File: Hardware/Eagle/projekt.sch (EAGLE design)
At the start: 141 parts, among them IC1 MEGA16-P, IC2 7805T, IC3 74LS157N, Q1 BC807-40SMD, Q10 2N2222, Q11 2N2222, Q12 2N2222, Q13 BC807-40SMD, Q14 BC807-40SMD, Q15 BC807-40SMD, Q16 BC807-40SMD, Q17 BC807-40SMD, Q18 BC807-40SMD, Q19 BC807-40SMD, Q2 BC807-40SMD, Q20 2N2222, Q22 2N2222, Q24 2N2222, Q26 2N2222, Q27 2N2222, Q29 2N2222, Q3 BC807-40SMD, Q30 2N2222, Q4 BC807-40SMD, Q5 BC807-40SMD, Q6 2N2222, Q7 2N2222, Q8 2N2222, Q9 2N2222

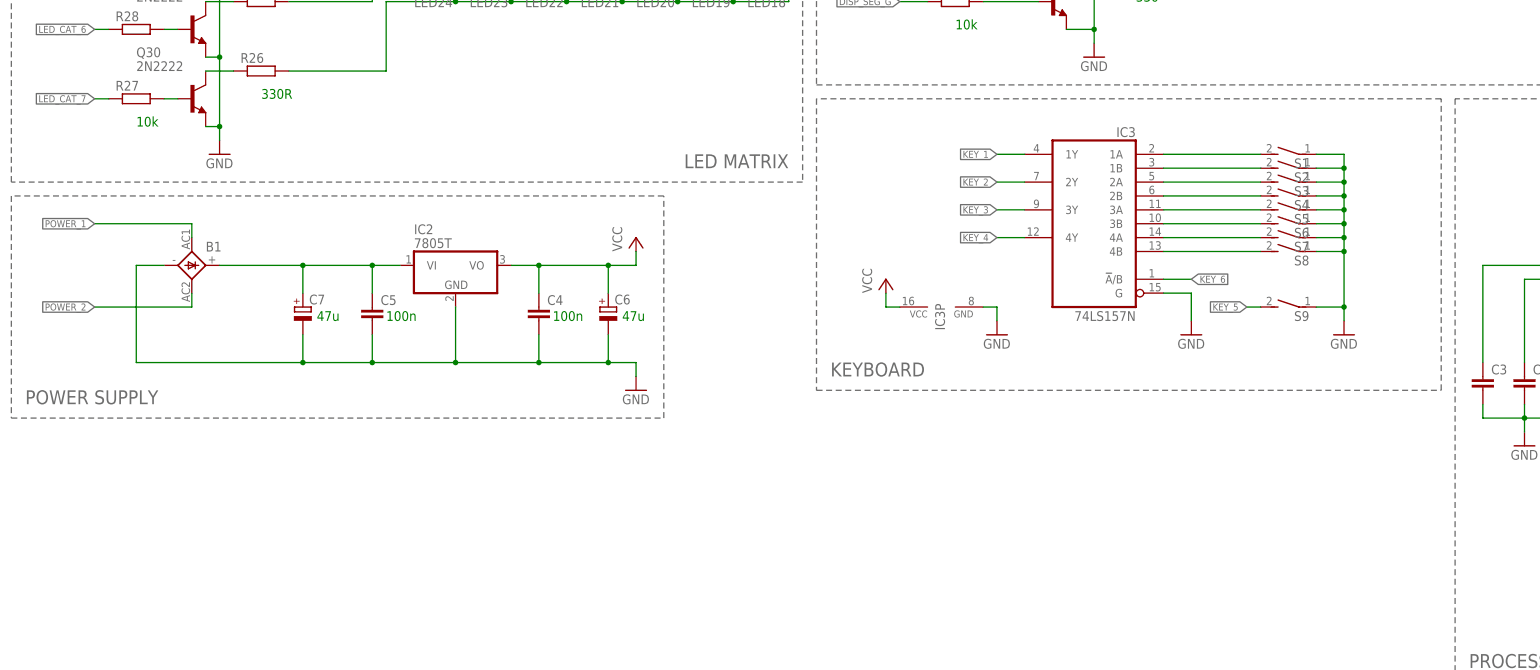
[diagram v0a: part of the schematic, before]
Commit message: przerwania, multiplekser
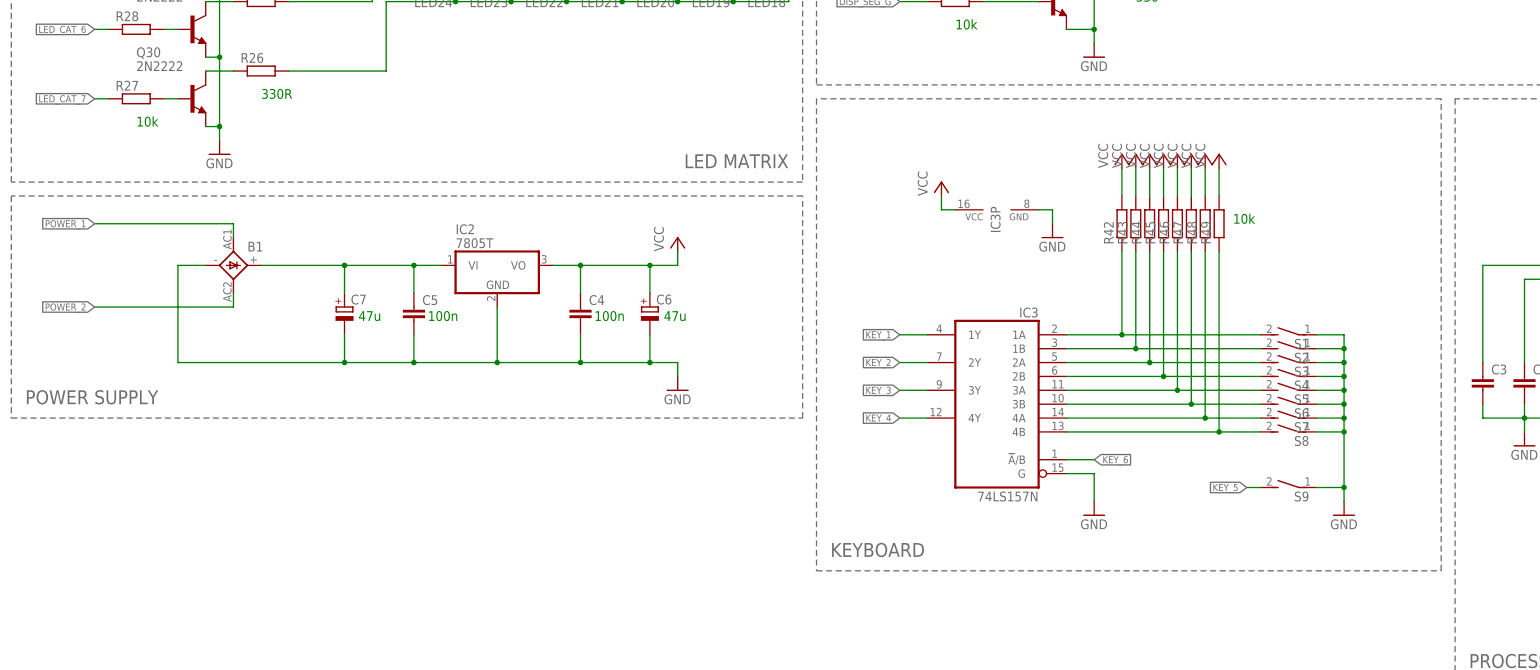
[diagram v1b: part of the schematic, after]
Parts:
- added R42, R43, R44, R45, R46, R47, R48, R49: (no value), resistor:R-EU_R0805
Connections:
- net N$27: now also R43.1
- net N$28: now also R44.1
- net N$29: now also R45.1
- net N$30: now also R46.1
- net N$31: now also R47.1
- net N$32: now also R48.1
- net N$33: now also R49.1
- net N$7: now also R42.1
- net VCC: now also R42.2, R43.2, R44.2, R45.2, R46.2, R47.2, R48.2, R49.2
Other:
- moved on the sheet: B1, C4, C5, C6, C7, IC2, IC3, IC3P, S1, S2, S3, S4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
